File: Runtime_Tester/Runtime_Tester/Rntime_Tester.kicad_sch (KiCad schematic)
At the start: 8 parts, among them IC1 RT9193-33GB, J1 USB1061-XX-X-X_REVA, U1 STM32F103C8Tx, U2 CAT24C256

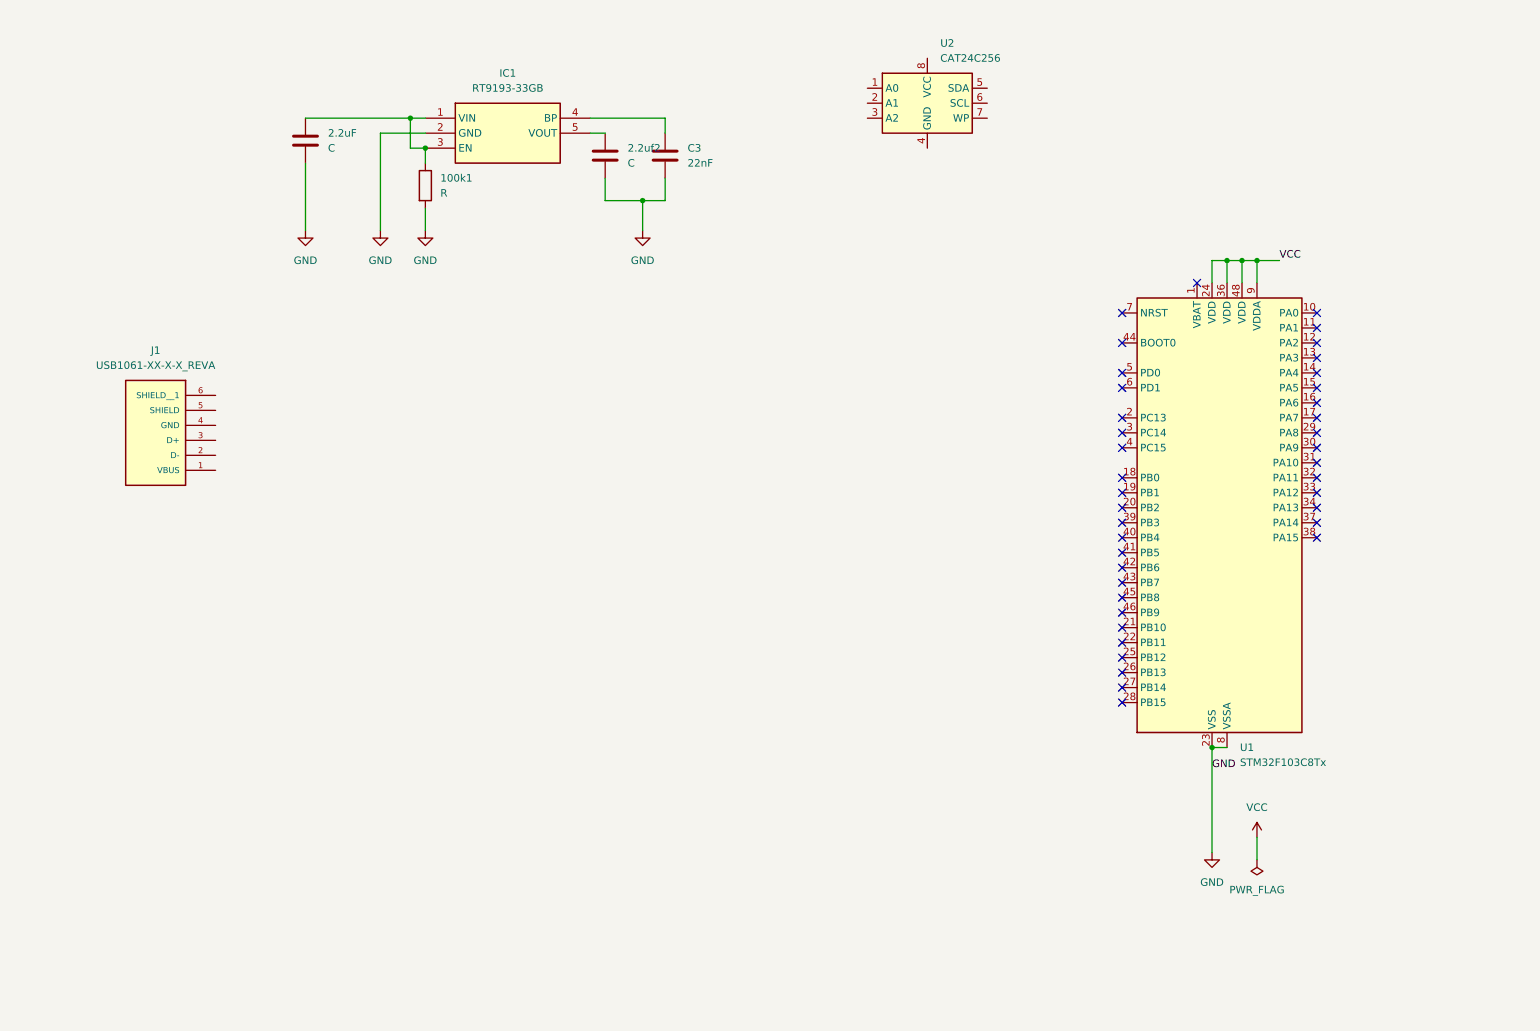
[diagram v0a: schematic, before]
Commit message: added more components
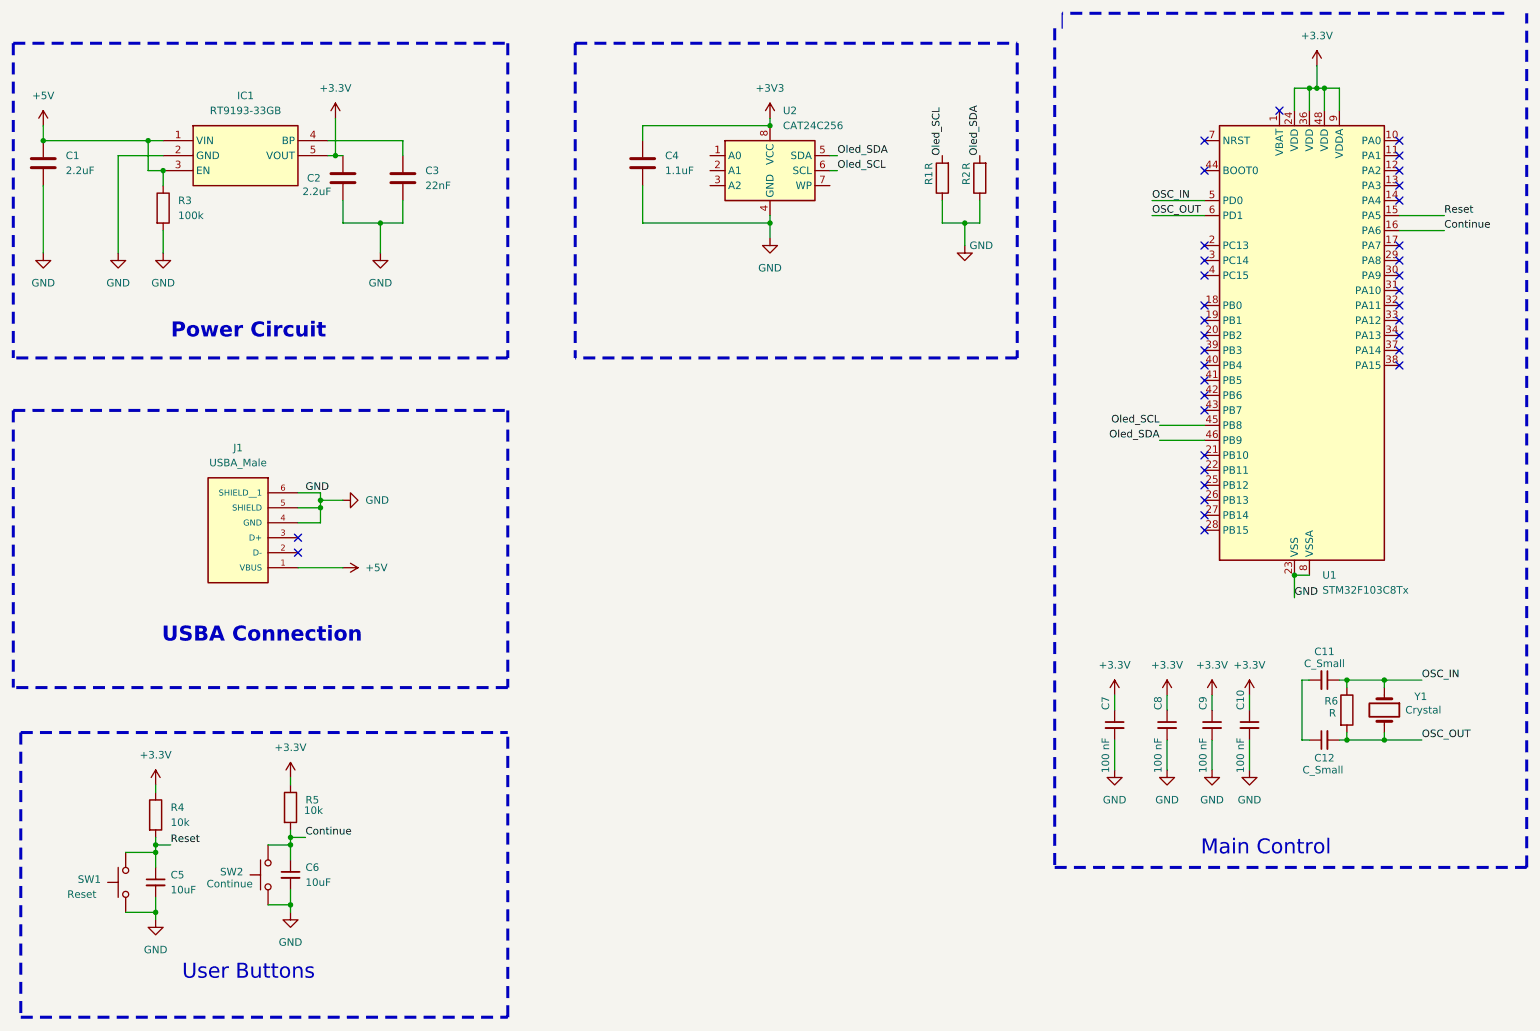
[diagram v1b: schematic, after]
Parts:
- added C10, C7, C8, C9: 100 nF, symbol Device:C_Small
- added C11, C12: C_Small, symbol Device:C_Small
- added C4: 1.1uF, Capacitor_SMD:C_0603_1608Metric, symbol Device:C
- added C5, C6: 10uF, symbol Device:C_Small
- added R1, R2, R6: R, symbol Device:R
- added R4, R5: 10k, symbol Device:R
- added SW1: Reset, symbol Switch:SW_Push
- added SW2: Continue, symbol Switch:SW_Push
- added Y1: Crystal, symbol Device:Crystal
- C1: renamed from 2.2uF; value C -> 2.2uF; footprint (none) -> Capacitor_SMD:C_0603_1608Metric
- C2: renamed from 2.2uf2; value C -> 2.2uF; footprint (none) -> Capacitor_SMD:C_0603_1608Metric
- C3: footprint (none) -> Capacitor_SMD:C_0603_1608Metric
- IC1: footprint SOT94P279X130-5N -> KiCad:SOT94P279X130-5N
- J1: value USB1061-XX-X-X_REVA -> USBA_Male
- R3: renamed from 100k1; value R -> 100k; footprint (none) -> Resistor_SMD:R_0603_1608Metric
- U2: footprint (none) -> 24C256:SOIC127P600X175-8N
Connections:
- net VCC is gone; now on net +3.3V: U1.24 (VDD), U1.36 (VDD), U1.48 (VDD), U1.9 (VDDA)
- net GND: now also J1.4 (GND), J1.5 (SHIELD), J1.6 (SHIELD__1), U2.4 (GND), C10.2, C4.2, C5.2, C6.2, C7.2, C8.2, C9.2, R1.1, R2.1, SW1.1, SW2.1
- net +3.3V: now reaches C2.1, IC1.5 (VOUT)
- net +3.3V: now also C10.1, C7.1, C8.1, C9.1, R4.1, R5.1
- net Oled_SDA: now reaches U2.5 (SDA)
- net Oled_SDA: now also U1.46 (PB9), R2.2
- net Oled_SCL: now reaches U2.6 (SCL)
- net Oled_SCL: now also U1.45 (PB8), R1.2
- net +3V3: now reaches U2.8 (VCC)
- net +3V3: now also C4.1
- net +5V: now reaches C1.1, IC1.1 (VIN), IC1.3 (EN), R3.1
- net +5V: now also J1.1 (VBUS)
- net Reset: now reaches U1.15 (PA5)
- net Reset: now also C5.1, R4.2, SW1.2
- net Continue: now reaches U1.16 (PA6)
- net Continue: now also C6.1, R5.2, SW2.2
- net OSC_IN: now reaches U1.5 (PD0)
- net OSC_IN: now also C11.1, R6.1, Y1.1
- net OSC_OUT: now reaches U1.6 (PD1)
- net OSC_OUT: now also C12.2, R6.2, Y1.2
- new net: C11.2, C12.1
- no-connect marks 40 -> 36
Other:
- note added: "Main Control"
- note added: "Power Circuit"
- note added: "USBA Connection"
- note added: "User Buttons"
- moved on the sheet: C1, C2, C3, IC1, J1, R3, U1, U2
